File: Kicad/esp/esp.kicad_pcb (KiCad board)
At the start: 2 copper layers, 44.4 x 68.2 mm, 42 parts, among them J1 Conn_01x19_Pin, J10 Sensor_car_out, J11 Sensor_gate_open, J12 Sensor_gate_close, J2 Conn_01x19_Pin, J3 LED_R, J4 LED_V, J5 SW_Open, J6 SW_Close, J7 Relay_gate_open, J8 Sensor_car_in, J9 Relay_gate_close, P1 USB_C_Plug_USB2.0, Q1 NPN, Q2 NPN, SW1 SW_Push, SW2 SW_Push, U1 AMS1117-3.3, U2 FT232RL, U3 ESP32-WROOM-E

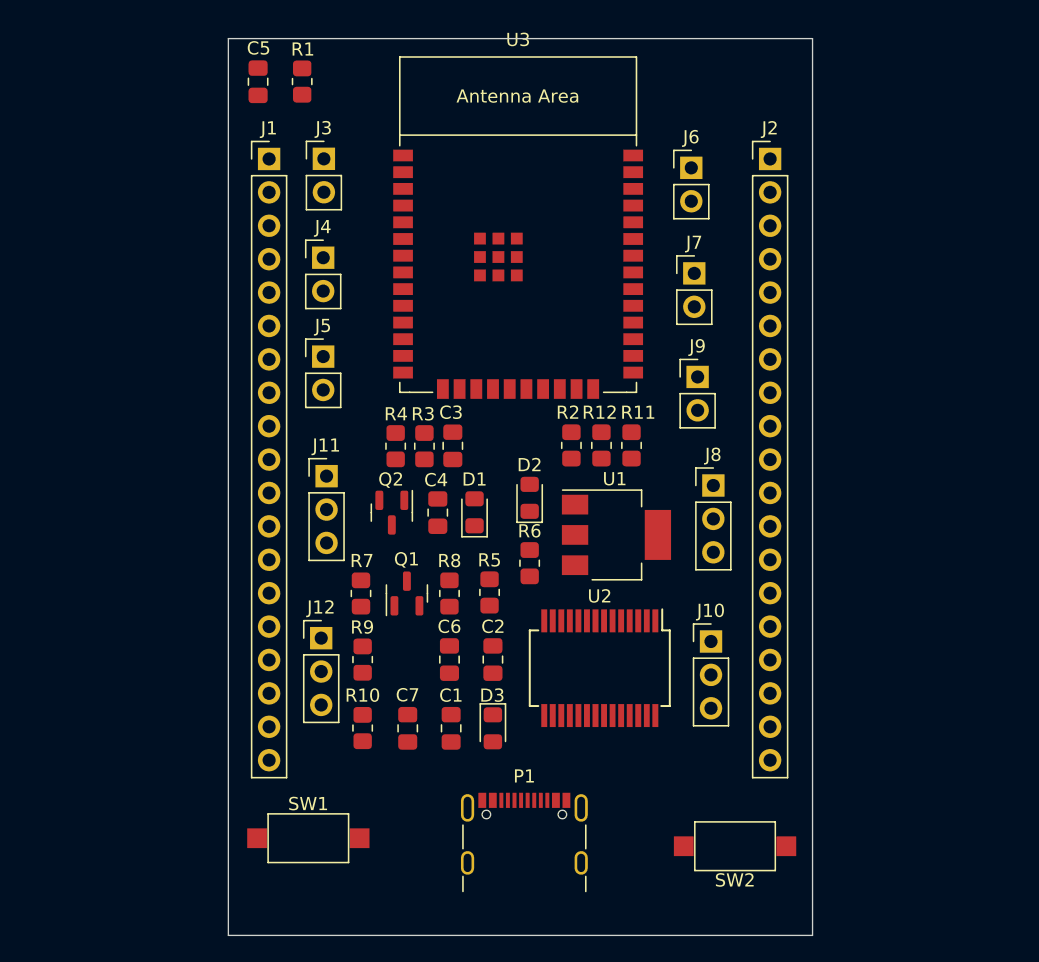
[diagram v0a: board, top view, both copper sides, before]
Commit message: Kicad Final
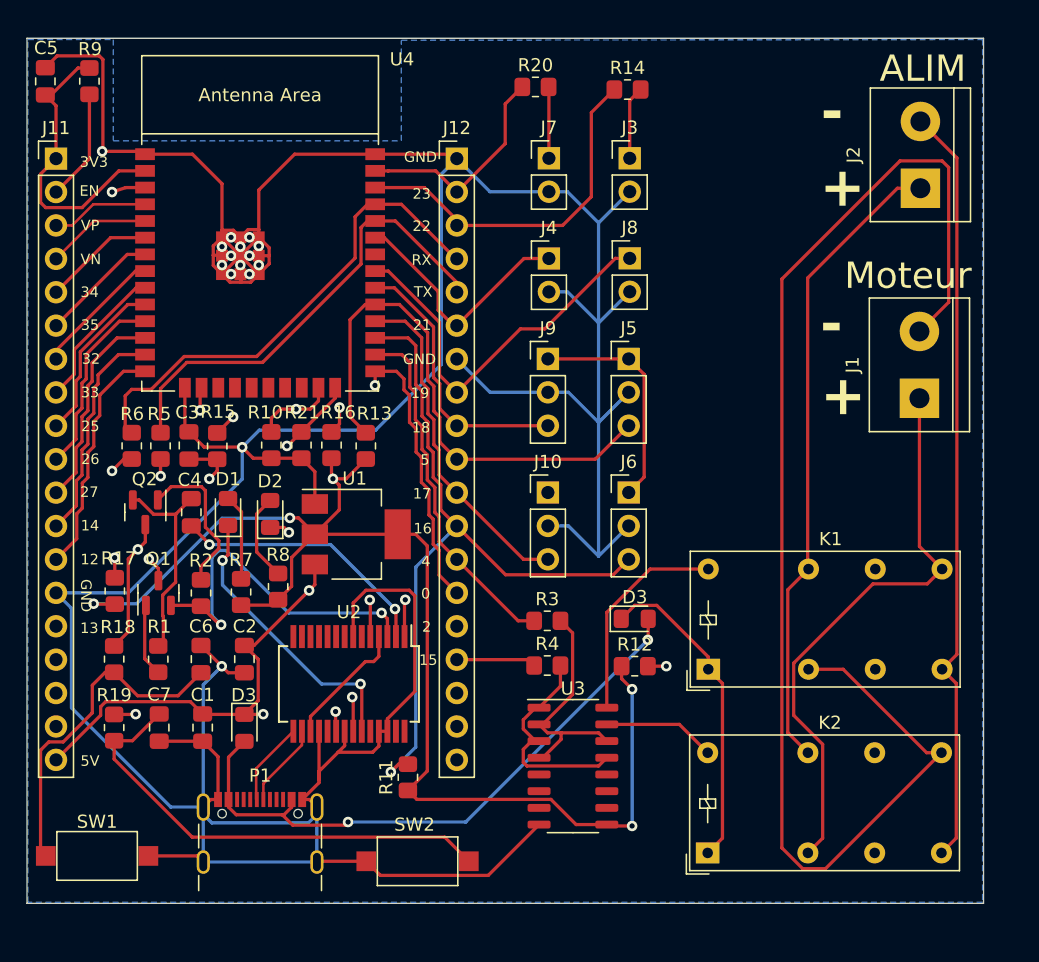
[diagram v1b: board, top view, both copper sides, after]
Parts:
- removed the J7 at (171.8, 78.2)
- removed the J9 at (172.0, 86.1)
- added D3: D_Schottky, Diode_SMD:D_0805_2012Metric_Pad1.15x1.40mm_HandSolder, F.Cu at (167.2, 104.5)
- added J1: ~, TerminalBlock:TerminalBlock_bornier-2_P5.08mm, F.Cu at (188.9, 87.7)
- added J2: ~, TerminalBlock:TerminalBlock_bornier-2_P5.08mm, F.Cu at (189.0, 71.7)
- added K1: FINDER-30.22, Relay_THT:Relay_DPDT_Finder_30.22, F.Cu at (172.8, 108.3)
- added K2: FINDER-30.22, Relay_THT:Relay_DPDT_Finder_30.22, F.Cu at (172.8, 122.3)
- added R11: 10K, Resistor_SMD:R_0805_2012Metric_Pad1.20x1.40mm_HandSolder, F.Cu at (150.0, 116.5)
- added R12: 10K, Resistor_SMD:R_0805_2012Metric_Pad1.20x1.40mm_HandSolder, F.Cu at (167.2, 108.0)
- added R13: 10K, Resistor_SMD:R_0805_2012Metric_Pad1.20x1.40mm_HandSolder, F.Cu at (146.8, 91.3)
- added R14: 300, Resistor_SMD:R_0805_2012Metric_Pad1.20x1.40mm_HandSolder, F.Cu at (166.7, 64.2)
- added R15: 10K, Resistor_SMD:R_0805_2012Metric_Pad1.20x1.40mm_HandSolder, F.Cu at (135.5, 91.3)
- added R17: 10K, Resistor_SMD:R_0805_2012Metric_Pad1.20x1.40mm_HandSolder, F.Cu at (127.7, 102.3)
- added R20: 300, Resistor_SMD:R_0805_2012Metric_Pad1.20x1.40mm_HandSolder, F.Cu at (159.7, 64.0)
- added R3: 220, Resistor_SMD:R_0805_2012Metric_Pad1.20x1.40mm_HandSolder, F.Cu at (160.6, 104.6)
- added R4: 220, Resistor_SMD:R_0805_2012Metric_Pad1.20x1.40mm_HandSolder, F.Cu at (160.6, 108.0)
- added U3: ULN2003, Package_SO:SO-16_3.9x9.9mm_P1.27mm, F.Cu at (162.6, 115.7)
- moved J9 24.8 mm to (160.6, 84.7)
- moved SW2 24.2 mm to (150.7, 122.9)
- moved J12 23.8 mm to (153.7, 69.5)
- moved J3 23.3 mm to (166.9, 69.4)
- moved J6 23.0 mm to (166.8, 94.8)
- moved R10 22.8 mm to (139.6, 91.2)
- moved R16 22.8 mm to (144.2, 91.2)
- moved R21 22.8 mm to (141.9, 91.2)
- moved J10 20.5 mm to (160.6, 94.8)
- moved P1 20.1 mm to (138.8, 121.9)
- moved R5 20.1 mm to (131.2, 91.3)
- moved R6 20.1 mm to (129.0, 91.3)
- moved C3 20.1 mm to (133.3, 91.3)
- moved U1 19.8 mm to (146.1, 98.0)
- moved D2 19.8 mm to (139.5, 96.5)
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- renumbered J12 to J10, J1 to J11, J2 to J12, J5 to J4, J8 to J5, J11 to J6, J4 to J7, J6 to J8, J10 to J9, R7 to R1, R2 to R10, R11 to R16, R9 to R18, R10 to R19, R8 to R2, R12 to R21, R3 to R5, R4 to R6, R5 to R7, R6 to R8, R1 to R9, U3 to U4
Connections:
- J10 pad 1: unconnected-(J12-Pin_1-Pad1) -> +5V
- J10 pad 2: unconnected-(J12-Pin_2-Pad2) -> GND
- J10 pad 3: unconnected-(J12-Pin_3-Pad3) -> /IO17
- J3 pad 1: unconnected-(J3-Pin_1-Pad1) -> Net-(J3-Pin_1)
- J3 pad 2: unconnected-(J3-Pin_2-Pad2) -> GND
- J4 pad 1: unconnected-(J5-Pin_1-Pad1) -> /IO21
- J4 pad 2: unconnected-(J5-Pin_2-Pad2) -> GND
- J5 pad 1: unconnected-(J8-Pin_1-Pad1) -> +5V
- J5 pad 2: unconnected-(J8-Pin_2-Pad2) -> GND
- J5 pad 3: unconnected-(J8-Pin_3-Pad3) -> /IO5
- J6 pad 1: unconnected-(J11-Pin_1-Pad1) -> +5V
- J6 pad 2: unconnected-(J11-Pin_2-Pad2) -> GND
- J6 pad 3: unconnected-(J11-Pin_3-Pad3) -> /IO16
- J7 pad 1: unconnected-(J4-Pin_1-Pad1) -> Net-(J7-Pin_1)
- J7 pad 2: unconnected-(J4-Pin_2-Pad2) -> GND
- J8 pad 1: unconnected-(J6-Pin_1-Pad1) -> /IO19
- J8 pad 2: unconnected-(J6-Pin_2-Pad2) -> GND
- J9 pad 1: unconnected-(J10-Pin_1-Pad1) -> +5V
- J9 pad 2: unconnected-(J10-Pin_2-Pad2) -> GND
- J9 pad 3: unconnected-(J10-Pin_3-Pad3) -> /IO18
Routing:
- net GND: track 0.00 -> 364.4 mm, vias 0 -> 15
- net +3.3V: track 0.00 -> 165.9 mm, vias 0 -> 6
- net +5V: track 0.00 -> 125.5 mm, vias 0 -> 3
- net Net-(J1-Pin_2): track 0.00 -> 102.4 mm
- net /EN: track 0.00 -> 69.9 mm, vias 0 -> 3
- net Net-(J2-Pin_2): track 0.00 -> 58.2 mm
- net /IO0: track 0.00 -> 58.0 mm, vias 0 -> 3
- net /IO16: track 0.00 -> 55.8 mm, vias 0 -> 1
- net /IO18: track 0.00 -> 55.7 mm, vias 0 -> 1
- net /IO21: track 0.00 -> 54.3 mm, vias 0 -> 1
- net Net-(J2-Pin_1): track 0.00 -> 48.8 mm
- net /IO17: track 0.00 -> 47.3 mm, vias 0 -> 1
- net Net-(D3-A): track 0.00 -> 46.9 mm, vias 0 -> 2
- net Net-(J1-Pin_1): track 0.00 -> 43.8 mm
- net /IO15: track 0.00 -> 42.7 mm, vias 0 -> 1
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- added copper zone on B.Cu, net GND
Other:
- board size 44.4 x 68.2 mm -> 72.7 x 65.8 mm
- copper layers 2 -> 4
- board text added: "+"
- board text added: "-"
- board text added: "0"
- board text added: "12"
- board text added: "13"
- board text added: "14"
- board text added: "15"
- board text added: "16"
- board text added: "17"
- board text added: "18"
- board text added: "19"
- board text added: "2"
- board text added: "21"
- board text added: "22"
- board text added: "23"
- board text added: "25"
- board text added: "26"
- board text added: "27"
- board text added: "32"
- board text added: "33"
- board text added: "34"
- board text added: "35"
- board text added: "3V3"
- board text added: "4"
- board text added: "5"
- board text added: "5V"
- board text added: "ALIM"
- board text added: "EN"
- board text added: "Etienne Dubé Mohammad Barin Wahidi"
- board text added: "GND"
- board text added: "Moteur"
- board text added: "RX"
- board text added: "TX"
- board text added: "VN"
- board text added: "VP"
